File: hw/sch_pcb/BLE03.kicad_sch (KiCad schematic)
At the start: 26 parts, among them J4 Conn_Coaxial, M1 HOLE, M2 HOLE, M3 HOLE, M4 HOLE, U1 CC3301, U6 LFB212G45CG1C187, Y1 TZ3877AAA044, Y2 LFSPXO009682

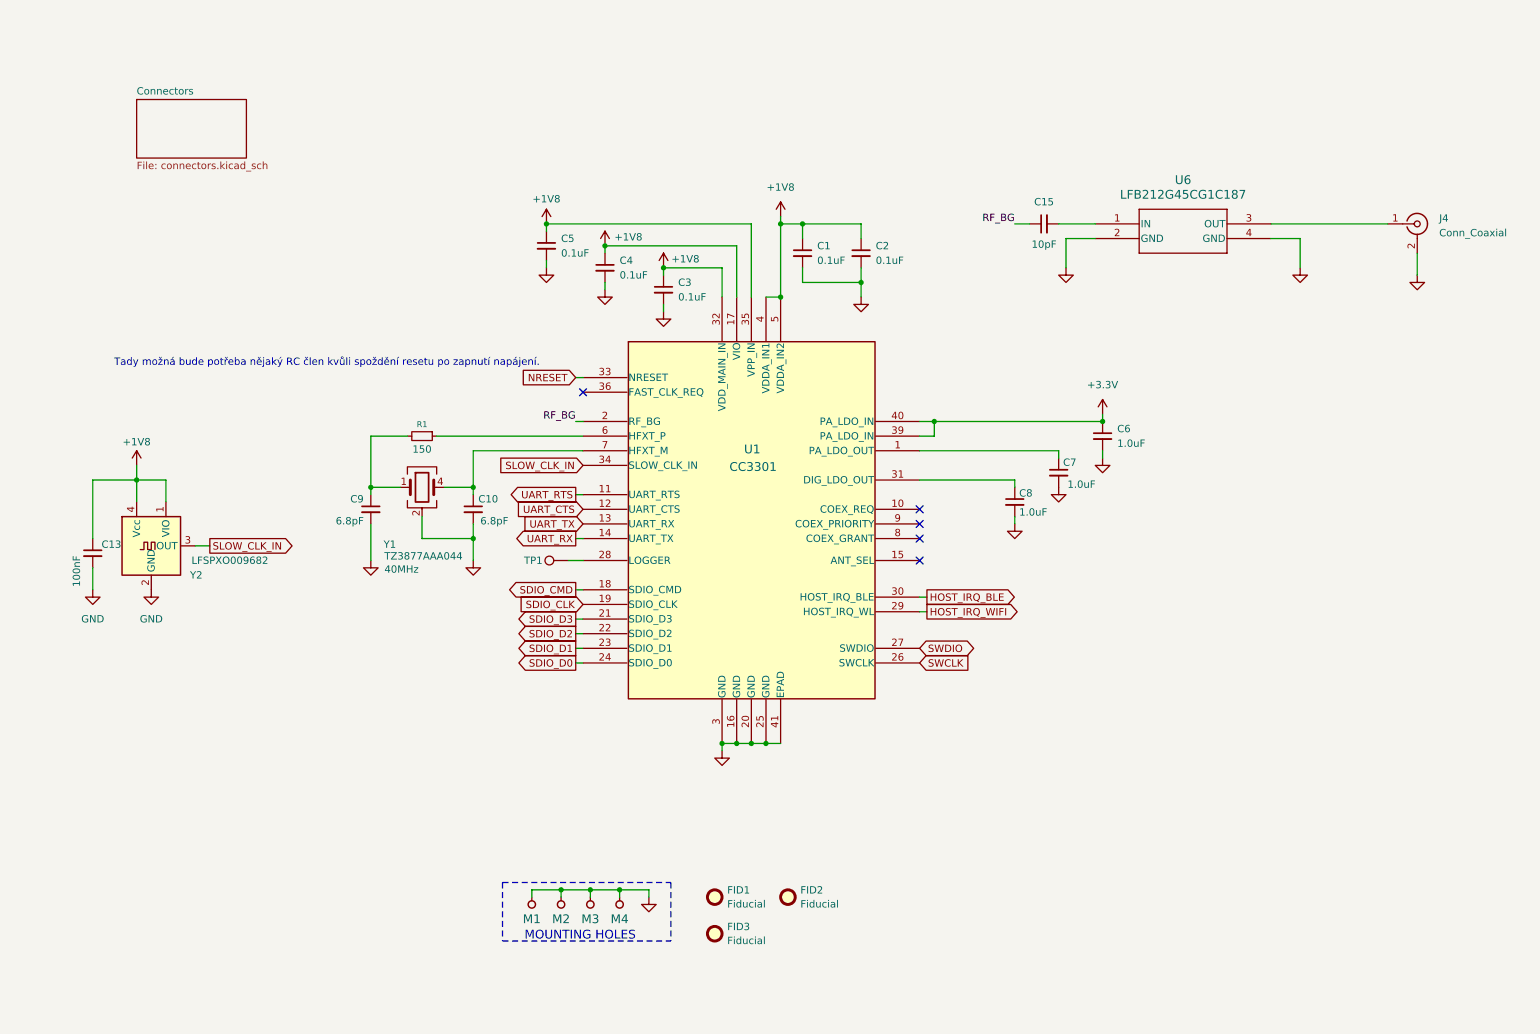
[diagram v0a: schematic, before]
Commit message: Adding connectors and other components
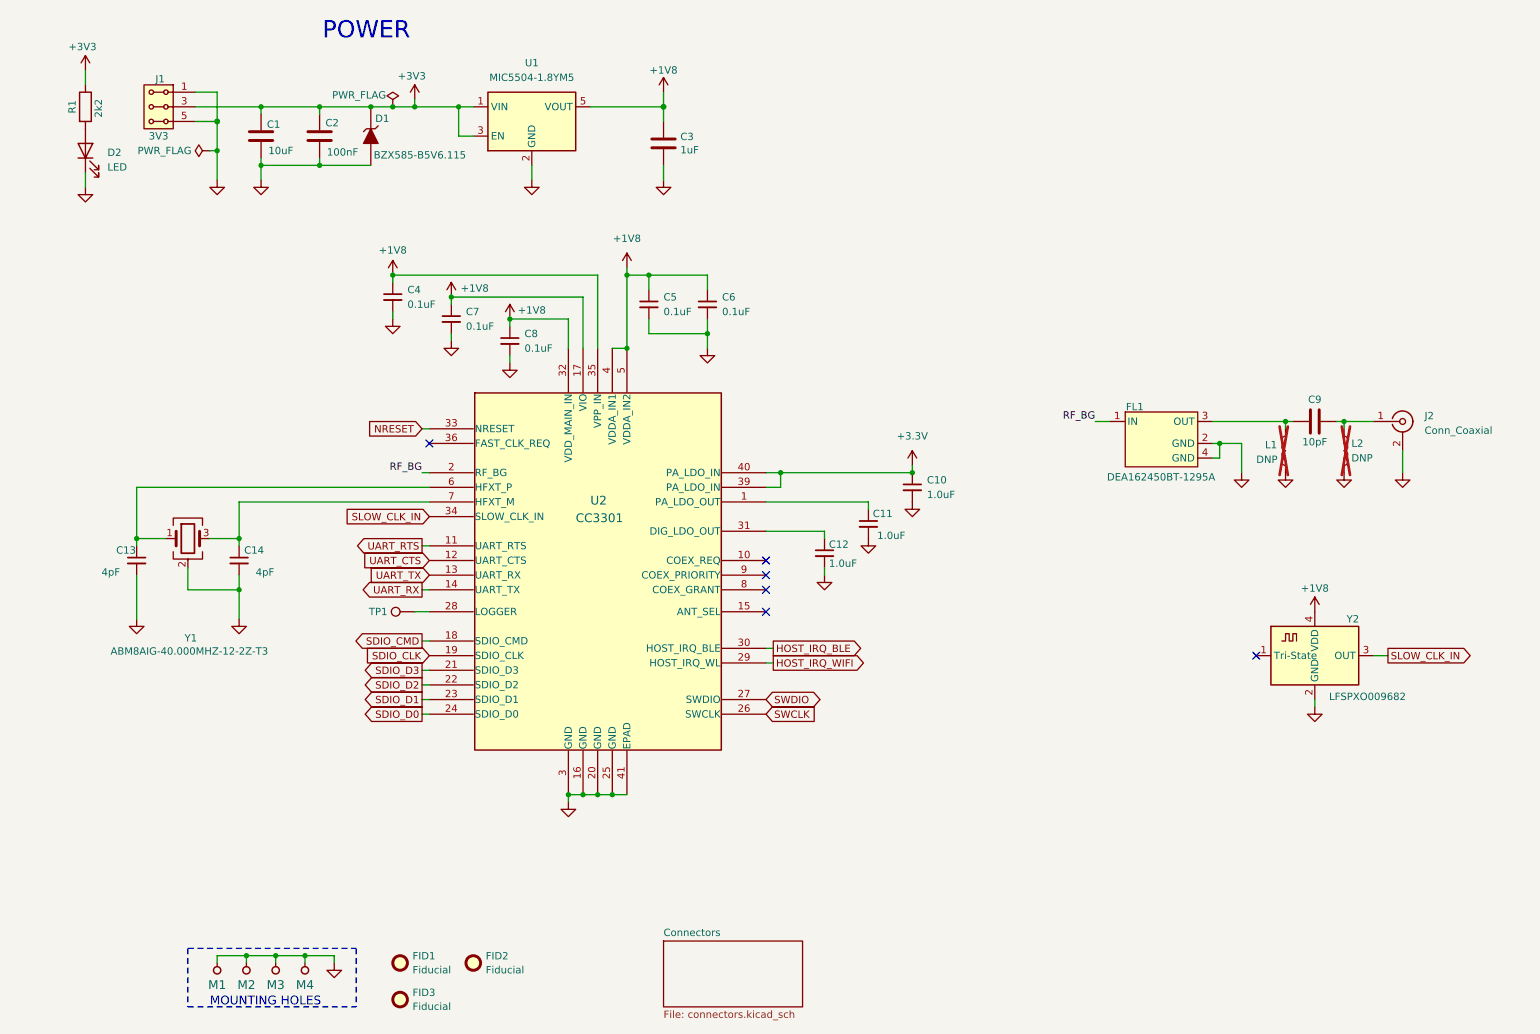
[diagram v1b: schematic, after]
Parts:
- removed C13: 100nF, Capacitor_SMD:C_0603_1608Metric, symbol Device:C_Small
- removed R1: 150, Resistor_SMD:R_0603_1608Metric, symbol Device:R_Small
- removed U6: LFB212G45CG1C187, MLAB_SAW:Murata_C187, symbol MLAB_Lib:LFB212G45CG1C187
- removed Y1: TZ3877AAA044, symbol Device:Crystal_GND23
- removed Y2: LFSPXO009682, Oscillator:Oscillator_SMD_SeikoEpson_SG210-4Pin_2.5x2.0mm, symbol Oscillator:SG-3030CM
- added C1: 10uF, Capacitor_SMD:C_0603_1608Metric, symbol Device:C
- added C2: 100nF, Capacitor_SMD:C_0603_1608Metric, symbol Device:C
- added C3: 1uF, Mlab_R:SMD-0603, symbol Device:C
- added D1: BZX585-B5V6.115, Diode_SMD:D_SOD-523, symbol MLAB_D:D_ZENER
- added D2: LED, LED_SMD:LED_0805_2012Metric, symbol Device:LED
- added FL1: DEA162450BT-1295A, Filter_custom:RF_1260B3_TDK, symbol BLE03_lib:DEA162450BT-1295A1
- added J1: 3V3, Mlab_Pin_Headers:Straight_2x03, symbol MLAB_HEADER:HEADER_2x03_PARALLEL
- added L1, L2: DNP, Inductor_SMD:L_0603_1608Metric, symbol Device:L
- added R1: 2k2, Resistor_SMD:R_0603_1608Metric, symbol cc2564-board-rescue:R-Device
- added U1: MIC5504-1.8YM5, Package_TO_SOT_SMD:SOT-23-5, symbol Regulator_Linear:MIC5504-1.8YM5
- added Y1: ABM8AIG-40.000MHZ-12-2Z-T3, Crystal:Crystal_SMD_Abracon_ABM8AIG-4Pin_3.2x2.5mm, symbol Device:Crystal_GND24
- added Y2: LFSPXO009682, Oscillator:Oscillator_SMD_Abracon_ASCO-4Pin_1.6x1.2mm, symbol Oscillator:ASCO
- C13: renamed from C9; value 6.8pF -> 4pF
- C14: renamed from C10; value 6.8pF -> 4pF
- C9: renamed from C15; symbol Device:C_Small -> Device:C
- TP1: footprint TestPoint:TestPoint_Pad_D1.0mm -> TestPoint:TestPoint_Pad_D1.5mm
- renumbered C6 to C10, C7 to C11, C8 to C12, C5 to C4, C1 to C5, C2 to C6, C4 to C7, C3 to C8, J4 to J2, U1 to U2
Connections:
- net +1V8: now also C3.1, U1.5 (VOUT), Y2.4 (VDD)
- net GND: now also C1.2, C2.2, C3.2, D1.2 (A), D2.1 (K), FL1.2 (GND), FL1.4 (GND), J1.1, J1.2, J1.5, J1.6, L1.1, L2.2, U1.2 (GND), Y1.2 (G), Y1.4 (G), Y2.2 (GND)
- net RF_BG: now also FL1.1 (IN); no longer C9.1
- net SLOW_CLK_IN: now also Y2.3 (OUT)
- net at J2.1 (In): now also C9.2, L2.1
- net at U2.6 (HFXT_P): now also C13.1, Y1.1
- net at C14.1, U2.7 (HFXT_M): now also Y1.3
- new net: C9.1, FL1.3 (OUT), L1.2
- new net: D2.2 (A), R1.2
- new net +3V3: C1.1, C2.1, D1.1 (K), J1.3, J1.4, R1.1, U1.1 (VIN), U1.3 (EN)
- no-connect marks 5 -> 6
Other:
- note added: "POWER"
- note removed: "Tady možná bude potřeba nějaký RC člen kvůli spoždění resetu po zapnutí napájení."
- moved on the sheet: C10, C11, C12, C13, C14, C4, C5, C6, C7, C8, C9, FID1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
